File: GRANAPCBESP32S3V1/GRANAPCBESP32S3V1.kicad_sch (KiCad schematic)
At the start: 3 parts, among them J1 Conn_01x14_Socket, P1 USB_C_Plug_USB2.0, U2 ESP32-S3-DevKitC

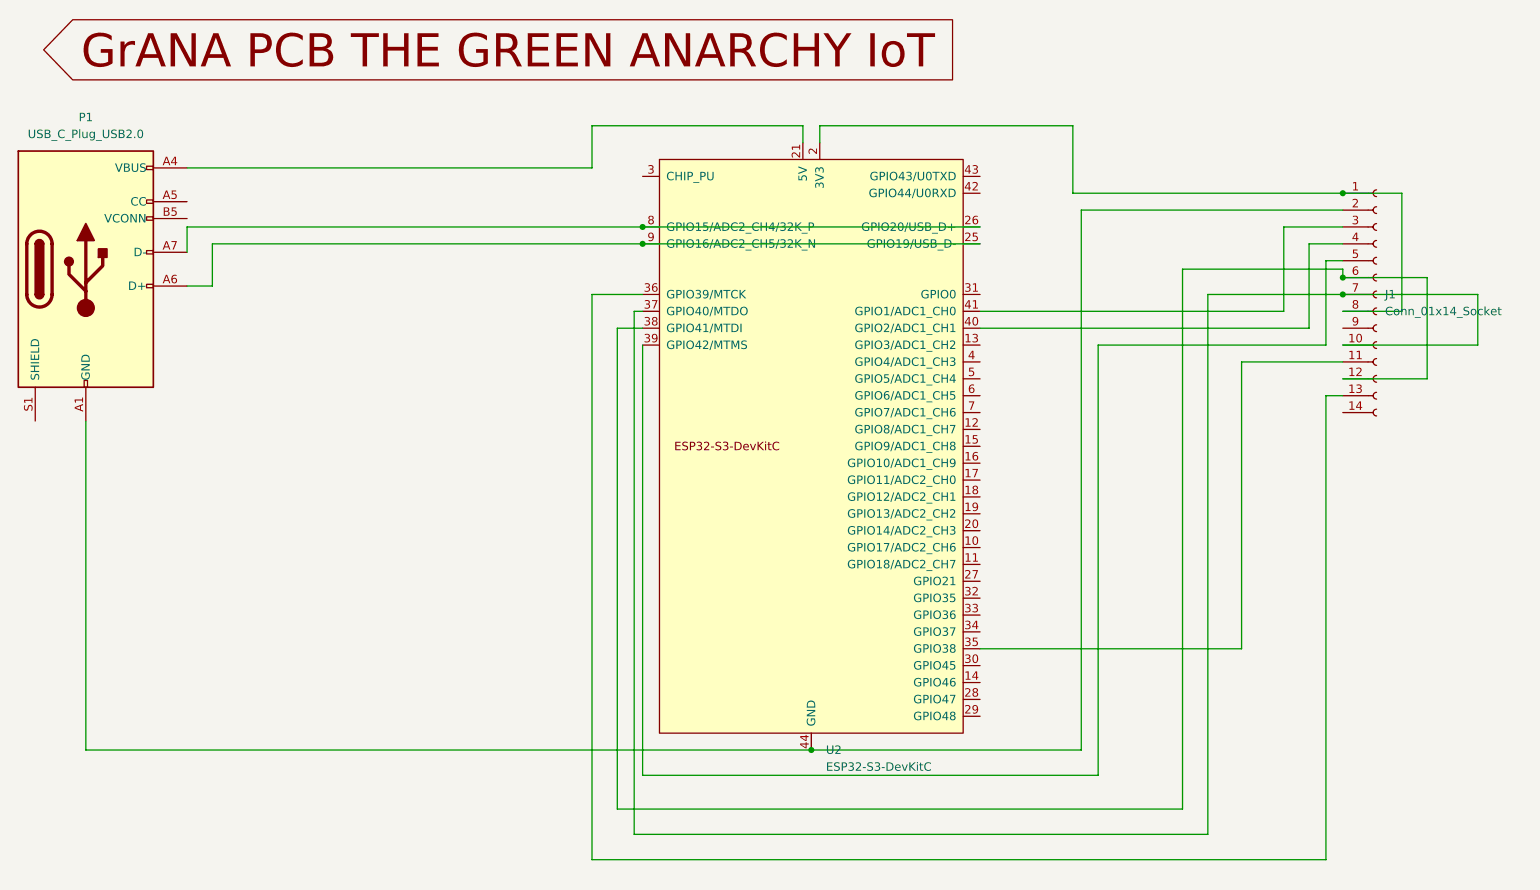
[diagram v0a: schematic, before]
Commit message: Add files via upload
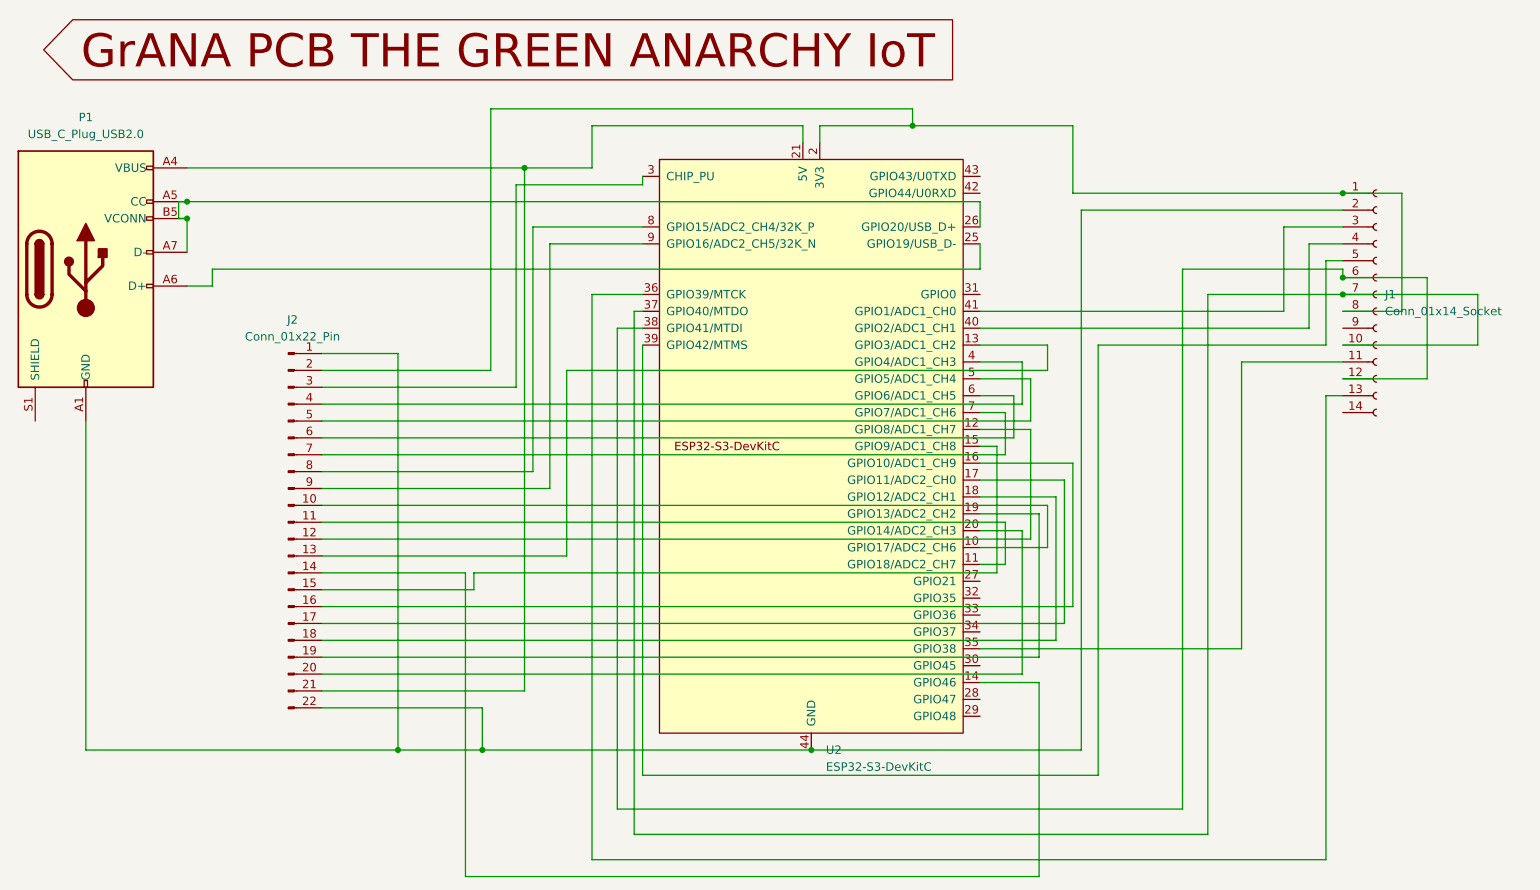
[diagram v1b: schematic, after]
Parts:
- added J2: Conn_01x22_Pin, Connector_PinSocket_2.54mm:PinSocket_1x22_P2.54mm_Vertical, symbol Connector:Conn_01x22_Pin
- J1: footprint (none) -> Connector_PinSocket_2.54mm:PinSocket_1x14_P2.54mm_Vertical
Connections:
- net at J1.1 (Pin_1), J1.8 (Pin_8), U2.1 (3V3)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: now also J2.2 (Pin_2)
- net at U2.10 (GPIO17/ADC2_CH6): now also J2.10 (Pin_10)
- net at U2.11 (GPIO18/ADC2_CH7): now also J2.11 (Pin_11)
- net at U2.12 (GPIO8/ADC1_CH7): now also J2.12 (Pin_12)
- net at U2.13 (GPIO3/ADC1_CH2): now also J2.13 (Pin_13)
- net at U2.14 (GPIO46): now also J2.14 (Pin_14)
- net at U2.15 (GPIO9/ADC1_CH8): now also J2.15 (Pin_15)
- net at U2.16 (GPIO10/ADC1_CH9): now also J2.16 (Pin_16)
- net at U2.17 (GPIO11/ADC2_CH0): now also J2.17 (Pin_17)
- net at U2.18 (GPIO12/ADC2_CH1): now also J2.18 (Pin_18)
- net at U2.19 (GPIO13/ADC2_CH2): now also J2.19 (Pin_19)
- net at U2.20 (GPIO14/ADC2_CH3): now also J2.20 (Pin_20)
- net at P1.A4 (VBUS), P1.A9 (VBUS), P1.B4 (VBUS)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: now also J2.21 (Pin_21)
- net at J1.2 (Pin_2), P1.A1 (GND), P1.A12 (GND)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: now also J2.1 (Pin_1), J2.22 (Pin_22)
- net at P1.A6 (D+), U2.25 (GPIO19/USB_D-): no longer U2.9 (GPIO16/ADC2_CH5/32K_N)
- net at P1.A7 (D-), U2.26 (GPIO20/USB_D+): now also P1.A5 (CC), P1.B5 (VCONN); no longer U2.8 (GPIO15/ADC2_CH4/32K_P)
- net at U2.3 (CHIP_PU): now also J2.3 (Pin_3)
- net at U2.4 (GPIO4/ADC1_CH3): now also J2.4 (Pin_4)
- net at U2.5 (GPIO5/ADC1_CH4): now also J2.5 (Pin_5)
- net at U2.6 (GPIO6/ADC1_CH5): now also J2.6 (Pin_6)
- net at U2.7 (GPIO7/ADC1_CH6): now also J2.7 (Pin_7)
- new net: J2.8 (Pin_8), U2.8 (GPIO15/ADC2_CH4/32K_P)
- new net: J2.9 (Pin_9), U2.9 (GPIO16/ADC2_CH5/32K_N)
